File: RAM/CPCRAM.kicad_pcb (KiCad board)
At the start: 2 copper layers, 99.1 x 52.9 mm, 20 parts, among them IC108 MC6845, IC110 74LS00, IC201 74LS157, IC202 74LS157, IC203 74LS157, IC204 74LS157, J1 Conn_01x16_Female, U191 AS6C4008-55PCN

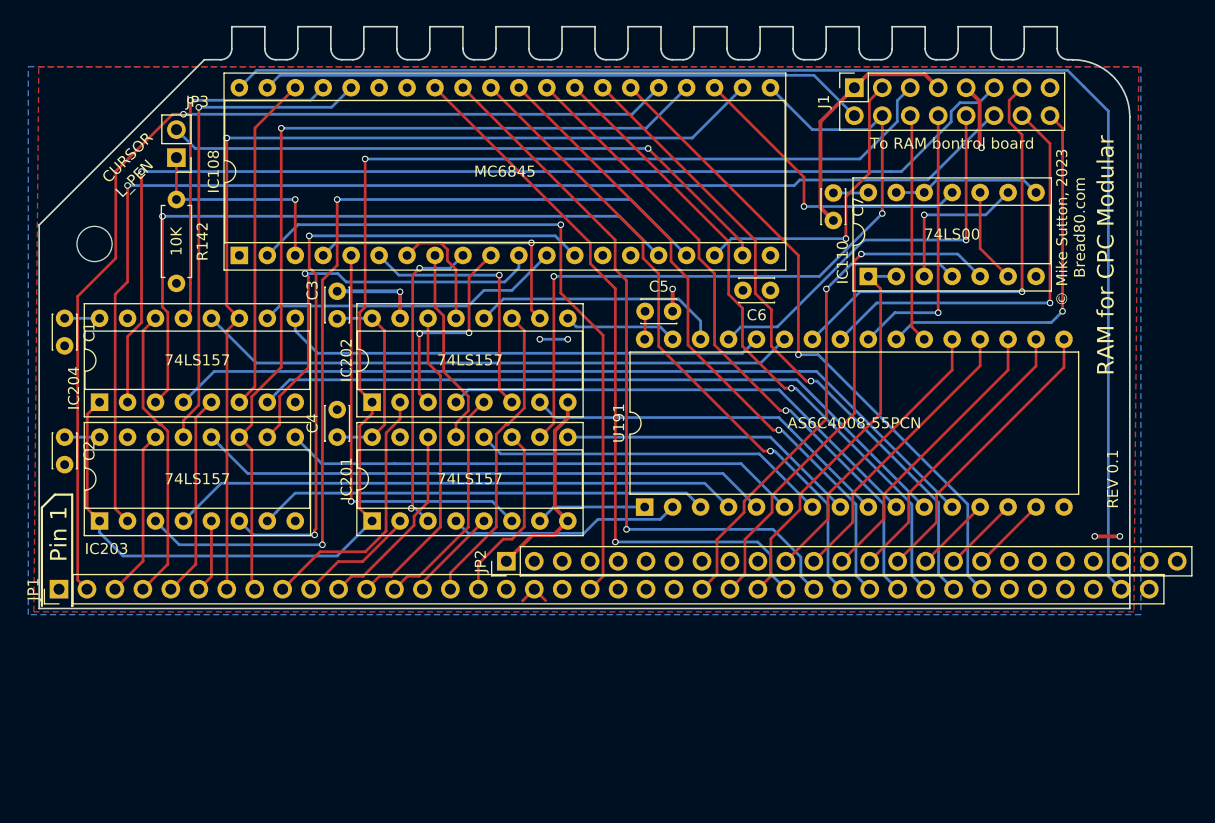
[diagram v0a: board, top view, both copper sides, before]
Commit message: Long overdue update...
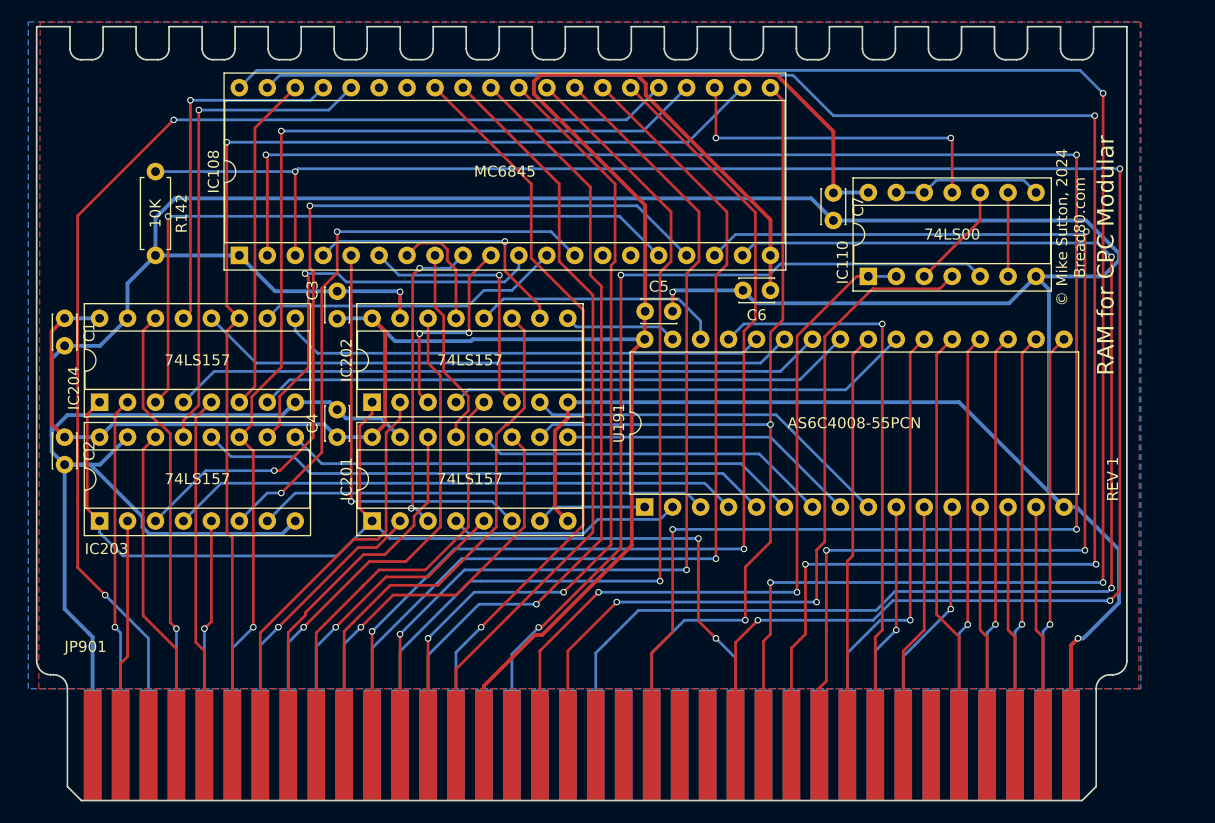
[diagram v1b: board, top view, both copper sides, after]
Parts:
- removed ?: , Mounting_Holes:MountingHole_3.2mm_M3
- removed J1: Conn_01x16_Female, Connector_PinSocket_2.54mm:PinSocket_2x08_P2.54mm_Vertical
- removed JP1: RC2014Bus, Connector_PinHeader_2.54mm:PinHeader_1x40_P2.54mm_Vertical
- removed JP3: Conn_01x02_Male, Connector_PinHeader_2.54mm:PinHeader_1x02_P2.54mm_Vertical
- added JP901: CPCM_VideoRAM_EdgeTop, CPCModular:Edge36_2.54PS, F.Cu at (158.8, 167.6)
- JP2: value RC2014ExtendedBus -> CPCM_VideoRAM_EdgeBottom; footprint Connector_PinHeader_2.54mm:PinHeader_1x25_P2.54mm_Vertical -> CPCModular:Edge36_2.54PS; moved to B.Cu
- moved JP2 40.4 mm to (158.8, 163.9), turned to 270 degrees
- moved R142 3.17 mm to (164.5, 113.7)
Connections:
- IC108 pad 40: /VSYNC -> /CRTC_ADDR_MULTI/VSYNC
- IC110 pad 3: Net-(IC110-Pad3) -> Net-(IC110-Pad10)
- IC110 pad 6: Net-(IC110-Pad10) -> Net-(IC110-Pad6)
- IC110 pad 9: Net-(IC110-Pad3) -> Net-(IC110-Pad6)
- JP2 pad 10: Net-(JP2-Pad10) -> A0
- JP2 pad 11: RAMD0 -> D6
- JP2 pad 12: RAMD1 -> D4
- JP2 pad 13: RAMD2 -> D2
- JP2 pad 14: RAMD3 -> D0
- JP2 pad 15: RAMD4 -> Net-(JP2-Pad15)
- JP2 pad 16: RAMD5 -> /CRTC_ADDR_MULTI/~RD
- JP2 pad 17: RAMD6 -> Net-(JP2-Pad17)
- JP2 pad 18: RAMD7 -> Net-(JP2-Pad18)
- JP2 pad 19: Net-(JP2-Pad19) -> /CRTC_ADDR_MULTI/CURSOR
- JP2 pad 2: +5V -> /CRTC_ADDR_MULTI/A14OUT
- JP2 pad 21: Net-(JP2-Pad21) -> /CRTC_ADDR_MULTI/MA0_CCLK
- JP2 pad 24: Net-(JP2-Pad24) -> /CRTC_ADDR_MULTI/~XCPU_ADDR
- JP2 pad 25: (no net) -> Net-(JP2-Pad25)
- JP2 pad 3: Net-(JP2-Pad3) -> A14
- JP2 pad 4: Net-(JP2-Pad4) -> A12
- JP2 pad 5: Net-(JP2-Pad5) -> A10
- JP2 pad 6: Net-(JP2-Pad6) -> A8
- JP2 pad 7: Net-(JP2-Pad7) -> A6
- JP2 pad 8: Net-(JP2-Pad8) -> A4
- JP2 pad 9: Net-(JP2-Pad9) -> A2
- U191 pad 10: RAMA7 -> RAMA18
- U191 pad 11: RAMA11 -> RAMA17
- U191 pad 12: RAMA14 -> RAMA16
- U191 pad 13: RAMD5 -> RD5
- U191 pad 14: RAMD6 -> RD3
- U191 pad 15: RAMD7 -> RD1
- U191 pad 17: RAMD4 -> RD0
- U191 pad 18: RAMD3 -> RD2
- U191 pad 19: RAMD2 -> RD4
- U191 pad 20: RAMD1 -> RD6
- U191 pad 21: RAMD0 -> RD7
- U191 pad 23: RAMA18 -> RAMA7
- U191 pad 25: RAMA17 -> RAMA11
- U191 pad 26: RAMA16 -> RAMA14
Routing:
- net GND: track 59.8 -> 395.6 mm, vias 5 -> 3
- net +5V: track 35.7 -> 221.8 mm, vias 2 -> 0
- net /CRTC_ADDR_MULTI/VSYNC: track 0.00 -> 171.6 mm, vias 0 -> 3
- net /CRTC_ADDR_MULTI/~L_PEN: track 19.7 -> 181.8 mm, vias 1 -> 4
- net /VSYNC: track 125.1 -> 0.00 mm
- net /CRTC_ADDR_MULTI/~RESET: track 63.0 -> 175.8 mm, vias 1 -> 4
- net /CRTC_ADDR_MULTI/HSYNC: track 55.3 -> 163.2 mm, vias 0 -> 3
- net /CRTC_ADDR_MULTI/A15OUT: track 112.8 -> 22.5 mm, vias 1 -> 0
- net /CRTC_ADDR_MULTI/DISPEN: track 27.7 -> 107.0 mm, vias 1 -> 3
- net /CRTC_ADDR_MULTI/A14OUT: track 102.7 -> 33.7 mm
- net /CRTC_ADDR_MULTI/CURSOR: track 56.8 -> 124.1 mm, vias 1 -> 2
- net RD7: track 0.00 -> 40.2 mm
- net RD6: track 0.00 -> 39.5 mm, vias 0 -> 1
- net RD4: track 0.00 -> 39.5 mm, vias 0 -> 1
- net RD2: track 0.00 -> 39.5 mm, vias 0 -> 1
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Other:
- board size 99.1 x 52.9 mm -> 99.1 x 70.3 mm
- board text added: "A modular Amstrad CPC compatible computer All capacitors are 0.1uF/100nF. Other values as marked. bread80.com - bread80@mstdn.social github.com/bread80"
- board text added: "REV 1"
- board text added: "© Mike Sutton, 2024 Bread80.com"
- board text removed: "A modular Amstrad CPC compatible using a (slightly modified) RC2014 backplace. This is NOT an RC2014 module. All capacitors are 0.1uF/100nF. Other values as marked. bread80.com - bread80@mstdn.social github.com/bread80 - twitter.com/bread80com"
- board text removed: "CURSOR"
- board text removed: "L_PEN"
- board text removed: "Pin 1"
- board text removed: "REV 0.1"
- board text removed: "To RAM bontrol board"
- board text removed: "© Mike Sutton, 2023 Bread80.com"
